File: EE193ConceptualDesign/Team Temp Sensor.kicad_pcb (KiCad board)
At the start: 2 copper layers, 48.9 x 62.2 mm, 33 parts, among them J1 USB_B_Micro, Q1 BC818, Q2 BC818, SW1 SW_DIP_x01, U1 ESP32-C3-WROOM-02, U2 CP2102N-A02-GQFN28, U3 LD1117S33TR_SOT223

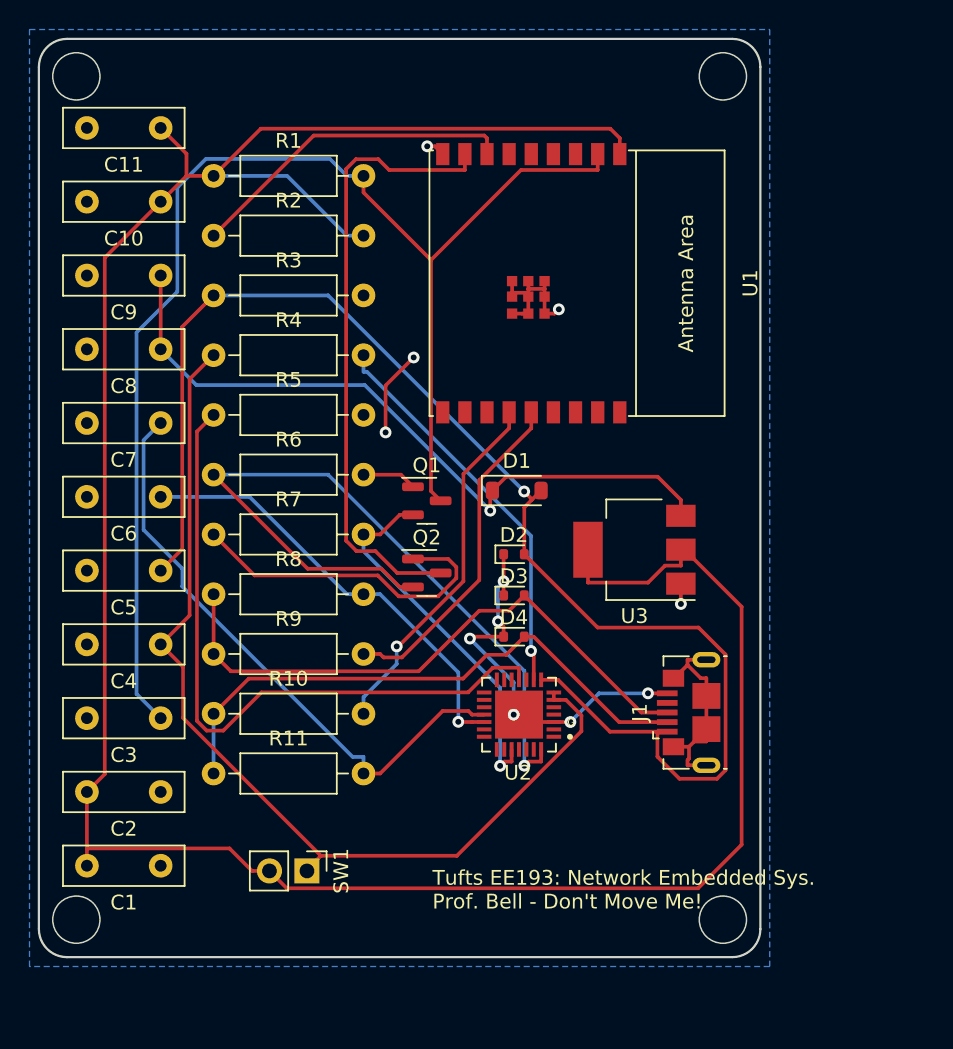
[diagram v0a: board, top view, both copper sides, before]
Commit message: new layout revision
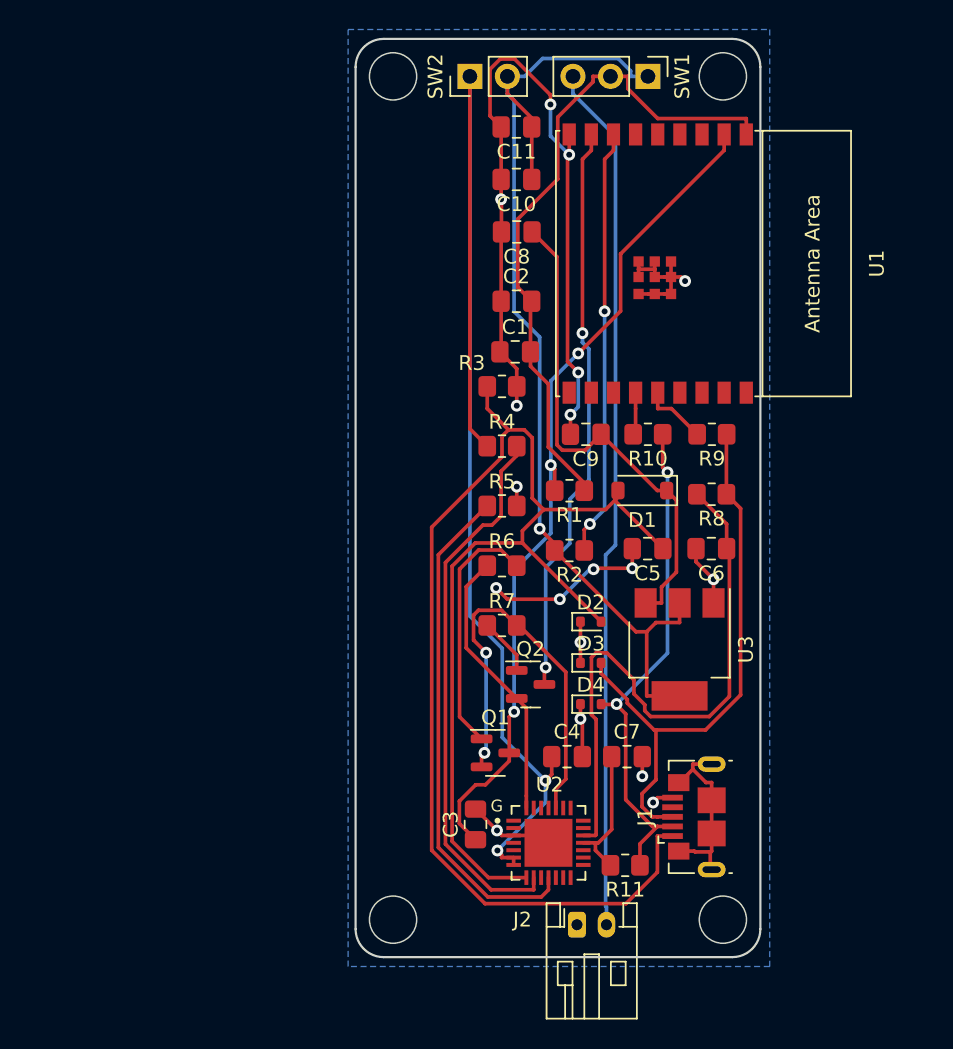
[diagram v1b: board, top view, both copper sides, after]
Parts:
- added J2: Battery_Connector, Connector_JST:JST_PH_S2B-PH-K_1x02_P2.00mm_Horizontal, F.Cu at (93.0, 111.5)
- added SW2: SW_DIP_x01, Connector_PinHeader_2.54mm:PinHeader_1x02_P2.54mm_Vertical, F.Cu at (85.7, 54.0)
- C1, C10, C11, C2, C3, C4, C5, C6, C7, C8, C9: footprint Capacitor_THT:C_Disc_D8.0mm_W2.5mm_P5.00mm -> Capacitor_SMD:C_0805_2012Metric_Pad1.18x1.45mm_HandSolder
- R1, R10, R11, R2, R3, R4, R5, R6, R7, R8, R9: footprint Resistor_THT:R_Axial_DIN0207_L6.3mm_D2.5mm_P10.16mm_Horizontal -> Resistor_SMD:R_0805_2012Metric_Pad1.20x1.40mm_HandSolder
- SW1: value SW_DIP_x01 -> SW_DPDT_x2; footprint Connector_PinHeader_2.54mm:PinHeader_1x02_P2.54mm_Vertical -> Connector_PinHeader_2.54mm:PinHeader_1x03_P2.54mm_Vertical
- moved SW1 58.6 mm to (97.8, 54.0)
- moved C1 42.3 mm to (88.8, 72.6), turned to 0 degrees
- moved C2 41.1 mm to (88.9, 69.2), turned to 0 degrees
- moved C7 38.9 mm to (96.4, 100.1), turned to 0 degrees
- moved C6 37.5 mm to (102.1, 86.0)
- moved R9 36.9 mm to (102.1, 78.2), turned to 180 degrees
- moved R10 35.0 mm to (97.8, 78.2), turned to 180 degrees
- moved R8 34.4 mm to (102.1, 82.3), turned to 180 degrees
- moved C5 33.0 mm to (97.8, 86.0)
- moved R1 32.2 mm to (92.5, 82.1), turned to 180 degrees
- moved R2 32.2 mm to (92.5, 86.1), turned to 180 degrees
- moved C9 30.8 mm to (93.6, 78.2)
- moved R11 28.6 mm to (96.2, 107.4), turned to 180 degrees
- moved C4 28.6 mm to (92.3, 100.1), turned to 0 degrees
- moved C8 25.4 mm to (88.9, 64.5)
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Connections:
- C1 pad 2: +3V3 -> PowerToESP32
- C2 pad 2: +3V3 -> PowerToESP32
- R1 pad 1: +3V3 -> PowerToESP32
- SW1 pad 1: Net-(U2-VDD) -> +3V3
- SW1 pad 2: +3V3 -> PowerToESP32
- U1 pad 1: +3V3 -> PowerToESP32
- U1 pad 5: unconnected-(U1-GPIO6-Pad5) -> SDA
- U1 pad 6: unconnected-(U1-GPIO7-Pad6) -> SCL
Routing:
- net +3V3: track 176.0 -> 70.8 mm, vias 0 -> 1
- net Net-(J2-Pin_2): track 0.00 -> 59.0 mm
- net GND: track 39.1 -> 96.6 mm, vias 9 -> 18
- net PowerToESP32: track 0.00 -> 45.3 mm
- net Net-(Q2-E): track 51.7 -> 18.7 mm, vias 1 -> 0
- net Net-(Q1-C): track 90.8 -> 57.9 mm, vias 0 -> 3
- net Net-(U2-GPIO.1/RXT): track 40.9 -> 9.18 mm
- net Net-(U1-GPIO18/USB_D-): track 24.6 -> 2.89 mm, vias 1 -> 0
- net Net-(D1-A): track 93.7 -> 113.3 mm, vias 1 -> 0
- net Net-(U2-VDD): track 66.4 -> 85.2 mm, vias 0 -> 2
- net Net-(Q2-B): track 22.6 -> 3.88 mm
- net Net-(U1-GPIO19/USB_D+): track 22.9 -> 4.47 mm
- net +5V: track 48.2 -> 34.1 mm, vias 1 -> 0
- net Net-(Q1-B): track 3.69 -> 17.0 mm
- net Net-(U2-~{SUSPEND}): track 45.9 -> 34.4 mm
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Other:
- board size 48.9 x 62.2 mm -> 27.4 x 62.2 mm
- board text added: "C10|10 uF"
- board text added: "C11|0.1 uF"
- board text added: "C1|10 uF"
- board text added: "C2|0.1 uF"
- board text added: "C4|10 uF"
- board text added: "C5|10 uF"
- board text added: "C6|22 pF"
- board text added: "C7|22 pF"
- board text added: "C8|10 uF"
- board text added: "C9|0.1 uF"
- board text added: "SW1|ESP32 Power"
- board text added: "SW2|UART Power"
- board text added: "||+3V3"
- board text added: "||Battery"
- board text added: "||To ESP32"
- board text removed: "Board By: Alex, Amitav, and Remy Board Revision: v0.1"
- board text removed: "C1 | 10 uF"
- board text removed: "C10 | 10 uF"
- board text removed: "C11 | 0.1 uF"
- board text removed: "C2 | 0.1 uF"
- board text removed: "C4 | 10 uF"
- board text removed: "C5 | 10 uF"
- board text removed: "C6 | 22 pF"
- board text removed: "C7 | 22 pF"
- board text removed: "C8 | 10 uF"
- board text removed: "C9 | 0.1 uF"
- board text removed: "Tufts EE193: Network Embedded Sys. Prof. Bell - Don't Move Me!"
